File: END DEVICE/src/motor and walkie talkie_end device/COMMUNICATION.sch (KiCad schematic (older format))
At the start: 20 parts, among them IC1 LM4871, J3 speaker_conn, U2 Ai-Thinker-Ra-02, U3 SA818-1W, U4 LP_Filter, U5 MCP41010

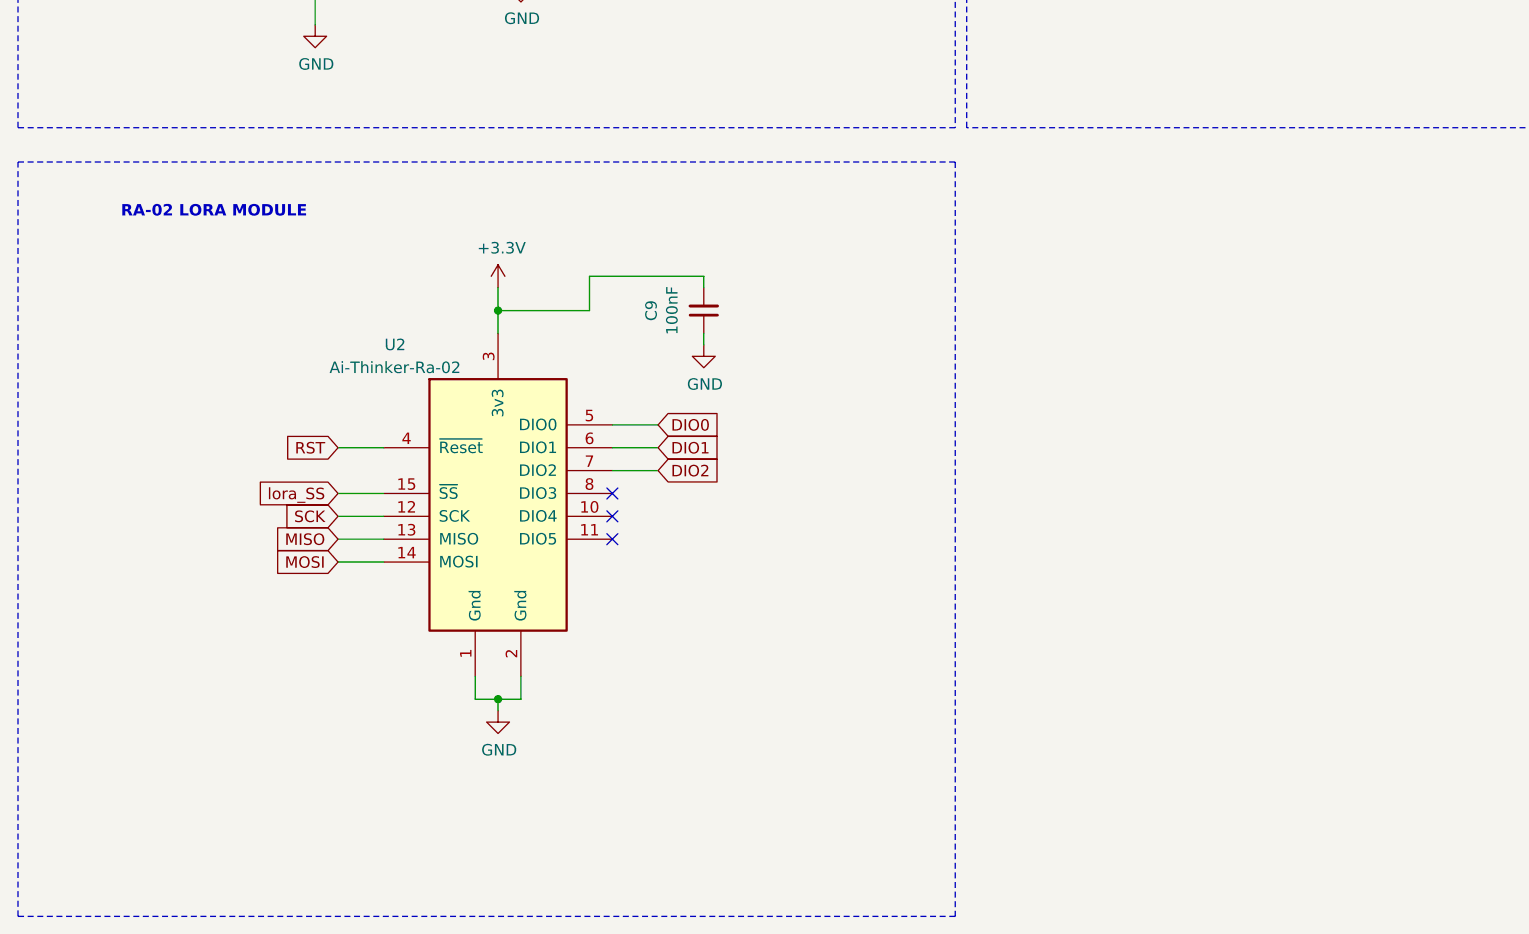
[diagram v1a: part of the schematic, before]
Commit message: third commit:very minor changes
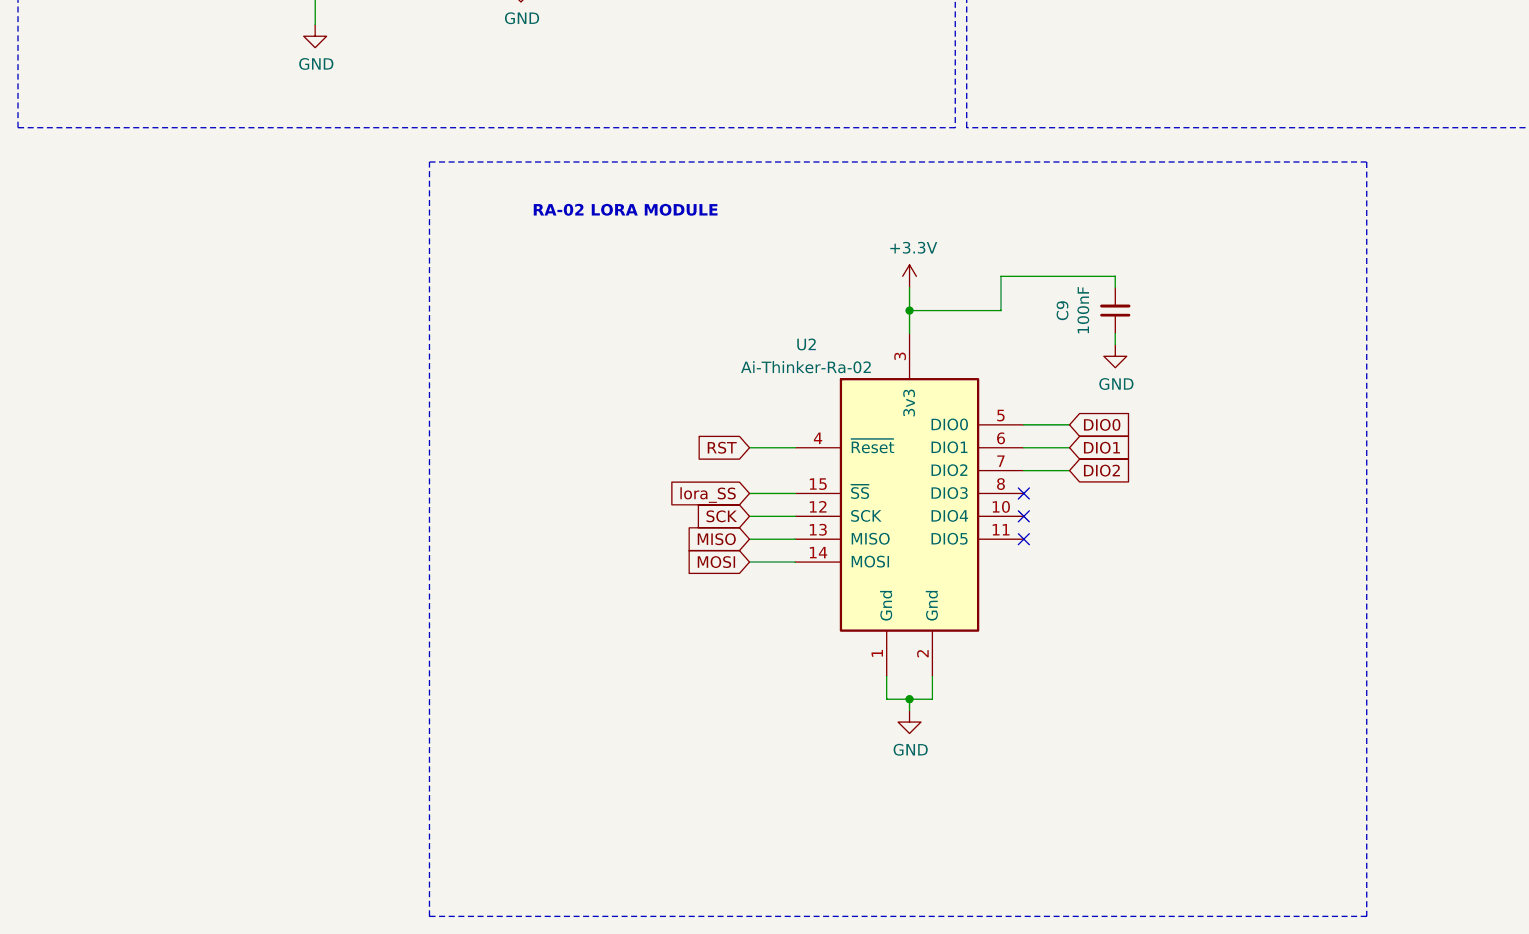
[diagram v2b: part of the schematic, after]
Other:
- moved on the sheet: C9, U2
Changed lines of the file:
@@
 Wire Wire Line
 	8300 2050 8300 1850
-Text GLabel 2000 6150 0    50   Input ~ 0
+Text GLabel 3800 6150 0    50   Input ~ 0
 MOSI
-Text GLabel 2000 6050 0    50   Input ~ 0
+Text GLabel 3800 6050 0    50   Input ~ 0
 MISO
-Text GLabel 2000 5950 0    50   Input ~ 0
+Text GLabel 3800 5950 0    50   Input ~ 0
 SCK
 $Comp
 L power:+3.3V #PWR0136
 U 1 1 614532C2
-P 2700 4950
-F 0 "#PWR0136" H 2700 4800 50  0001 C CNN
-F 1 "+3.3V" H 2715 5123 50  0000 C CNN
-F 2 "" H 2700 4950 50  0001 C CNN
-F 3 "" H 2700 4950 50  0001 C CNN
-	1    2700 4950
+P 4500 4950
+F 0 "#PWR0136" H 4500 4800 50  0001 C CNN
+F 1 "+3.3V" H 4515 5123 50  0000 C CNN
+F 2 "" H 4500 4950 50  0001 C CNN
+F 3 "" H 4500 4950 50  0001 C CNN
+	1    4500 4950
 	1    0    0    -1
 $EndComp
 Wire Wire Line
-	2200 6150 2000 6150
+	4000 6150 3800 6150
 Wire Wire Line
-	2000 6050 2200 6050
+	3800 6050 4000 6050
 Wire Wire Line
-	2200 5950 2000 5950
+	4000 5950 3800 5950
 Wire Wire Line
-	2000 5850 2200 5850
+	3800 5850 4000 5850
 Wire Wire Line
-	2200 5650 2000 5650
+	4000 5650 3800 5650
 $Comp
 L Device:C_Small C?
 U 1 1 614532CD
-P 3600 5050
+P 5400 5050
 AR Path="/614532CD" Ref="C?"  Part="1"
 AR Path="/6131B829/614532CD" Ref="C9"  Part="1"
-F 0 "C9" V 3829 5050 50  0000 C CNN
-F 1 "100nF" V 3738 5050 50  0000 C CNN
-F 2 "" H 3600 5050 50  0001 C CNN
-F 3 "~" H 3600 5050 50  0001 C CNN
-	1    3600 5050
+F 0 "C9" V 5629 5050 50  0000 C CNN
+F 1 "100nF" V 5538 5050 50  0000 C CNN
+F 2 "" H 5400 5050 50  0001 C CNN
+F 3 "~" H 5400 5050 50  0001 C CNN
+	1    5400 5050
 	-1   0    0    1
 $EndComp
@@
 L remote_devices:Ai-Thinker-Ra-02 U?
 U 1 1 614532D3
-P 2700 5950
+P 4500 5950
 AR Path="/614532D3" Ref="U?"  Part="1"
 AR Path="/6131B829/614532D3" Ref="U2"  Part="1"
-F 0 "U2" H 2250 6700 50  0000 C CNN
-F 1 "Ai-Thinker-Ra-02" H 2250 6600 50  0000 C CNN
-F 2 "Remote_devices:Ai-Thinker-Ra-02-LoRa" H 3700 5550 50  0001 C CNN
-F 3 "https://mikroelectron.com/Product/10KM-433M-LORA-LONG-RANGE-WIRELESS-MODULE-RA-01" H 2800 6650 50  0001 C CNN
-	1    2700 5950
+F 0 "U2" H 4050 6700 50  0000 C CNN
+F 1 "Ai-Thinker-Ra-02" H 4050 6600 50  0000 C CNN
+F 2 "Remote_devices:Ai-Thinker-Ra-02-LoRa" H 5500 5550 50  0001 C CNN
+F 3 "https://mikroelectron.com/Product/10KM-433M-LORA-LONG-RANGE-WIRELESS-MODULE-RA-01" H 4600 6650 50  0001 C CNN
+	1    4500 5950
 	1    0    0    -1
 $EndComp
 Wire Wire Line
-	3600 4900 3600 4950
+	5400 4900 5400 4950
 $Comp
 L power:GND #PWR0137
 U 1 1 614532DA
-P 3600 5200
-F 0 "#PWR0137" H 3600 4950 50  0001 C CNN
-F 1 "GND" H 3605 5027 50  0000 C CNN
-F 2 "" H 3600 5200 50  0001 C CNN
-F 3 "" H 3600 5200 50  0001 C CNN
-	1    3600 5200
+P 5400 5200
+F 0 "#PWR0137" H 5400 4950 50  0001 C CNN
+F 1 "GND" H 5405 5027 50  0000 C CNN
+F 2 "" H 5400 5200 50  0001 C CNN
+F 3 "" H 5400 5200 50  0001 C CNN
+	1    5400 5200
 	1    0    0    -1
 $EndComp
@@
 L power:GND #PWR0138
 U 1 1 614532E0
-P 2700 6800
-F 0 "#PWR0138" H 2700 6550 50  0001 C CNN
-F 1 "GND" H 2705 6627 50  0000 C CNN
-F 2 "" H 2700 6800 50  0001 C CNN
-F 3 "" H 2700 6800 50  0001 C CNN
-	1    2700 6800
+P 4500 6800
+F 0 "#PWR0138" H 4500 6550 50  0001 C CNN
+F 1 "GND" H 4505 6627 50  0000 C CNN
+F 2 "" H 4500 6800 50  0001 C CNN
+F 3 "" H 4500 6800 50  0001 C CNN
+	1    4500 6800
 	1    0    0    -1
 $EndComp
 Wire Wire Line
-	2700 6800 2700 6750
+	4500 6800 4500 6750
 Wire Wire Line
-	2600 6650 2600 6750
+	4400 6650 4400 6750
 Wire Wire Line
-	2600 6750 2700 6750
+	4400 6750 4500 6750
 Wire Wire Line
-	2800 6650 2800 6750
+	4600 6650 4600 6750
 Wire Wire Line
-	2800 6750 2700 6750
-Connection ~ 2700 6750
-Text GLabel 3400 5550 2    50   Input ~ 0
+	4600 6750 4500 6750
+Connection ~ 4500 6750
+Text GLabel 5200 5550 2    50   Input ~ 0
 DIO0
 Wire Wire Line
-	2700 4950 2700 5050
+	4500 4950 4500 5050
 Wire Wire Line
-	3600 5200 3600 5150
+	5400 5200 5400 5150
 Wire Wire Line
-	3600 4900 3100 4900
+	5400 4900 4900 4900
 Wire Wire Line
-	3100 4900 3100 5050
+	4900 4900 4900 5050
 Wire Wire Line
-	3100 5050 2700 5050
-Connection ~ 2700 5050
+	4900 5050 4500 5050
+Connection ~ 4500 5050
 Wire Wire Line
-	2700 5050 2700 5150
-Text GLabel 3400 5650 2    50   Input ~ 0
+	4500 5050 4500 5150
+Text GLabel 5200 5650 2    50   Input ~ 0
 DIO1
-Text GLabel 3400 5750 2    50   Input ~ 0
+Text GLabel 5200 5750 2    50   Input ~ 0
 DIO2
 Wire Wire Line
-	3200 5550 3400 5550
+	5000 5550 5200 5550
 Wire Wire Line
-	3400 5650 3200 5650
+	5200 5650 5000 5650
 Wire Wire Line
-	3200 5750 3400 5750
-NoConn ~ 3200 5850
-NoConn ~ 3200 5950
-NoConn ~ 3200 6050
-Text Notes 1050 4650 0    50   ~ 10
+	5000 5750 5200 5750
+NoConn ~ 5000 5850
+NoConn ~ 5000 5950
+NoConn ~ 5000 6050
+Text Notes 2850 4650 0    50   ~ 10
 RA-02 LORA MODULE
 Wire Notes Line
-	4700 4400 4700 7700
+	6500 4400 6500 7700
 Wire Notes Line
-	4700 7700 600  7700
+	6500 7700 2400 7700
 Wire Notes Line
-	600  7700 600  4400
+	2400 7700 2400 4400
 Wire Notes Line
 	10850 2500 10850 2750
@@
 Text Notes 6150 3300 0    50   ~ 0
 Digital Potentiometer uses \nSPI protocol to change resistance\nused for setting the volume of the speaker
-Text GLabel 2000 5850 0    50   Input ~ 0
+Text GLabel 3800 5850 0    50   Input ~ 0
 lora_SS
 Text GLabel 5600 2300 0    50   Input ~ 0
@@
 Wire Notes Line
 	1150 2650 1200 2650
-Text GLabel 2000 5650 0    50   Input ~ 0
+Text GLabel 3800 5650 0    50   Input ~ 0
 RST
 Wire Notes Line
-	600  4400 4700 4400
+	2400 4400 6500 4400
 Wire Notes Line
 	4700 4250 600  4250
